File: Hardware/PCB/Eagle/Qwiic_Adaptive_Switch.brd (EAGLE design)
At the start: 41.9 x 30.5 mm, 18 parts, among them J2 J2, SW1 CUI_SJ1-3513, SW2 CUI_SJ1-3513

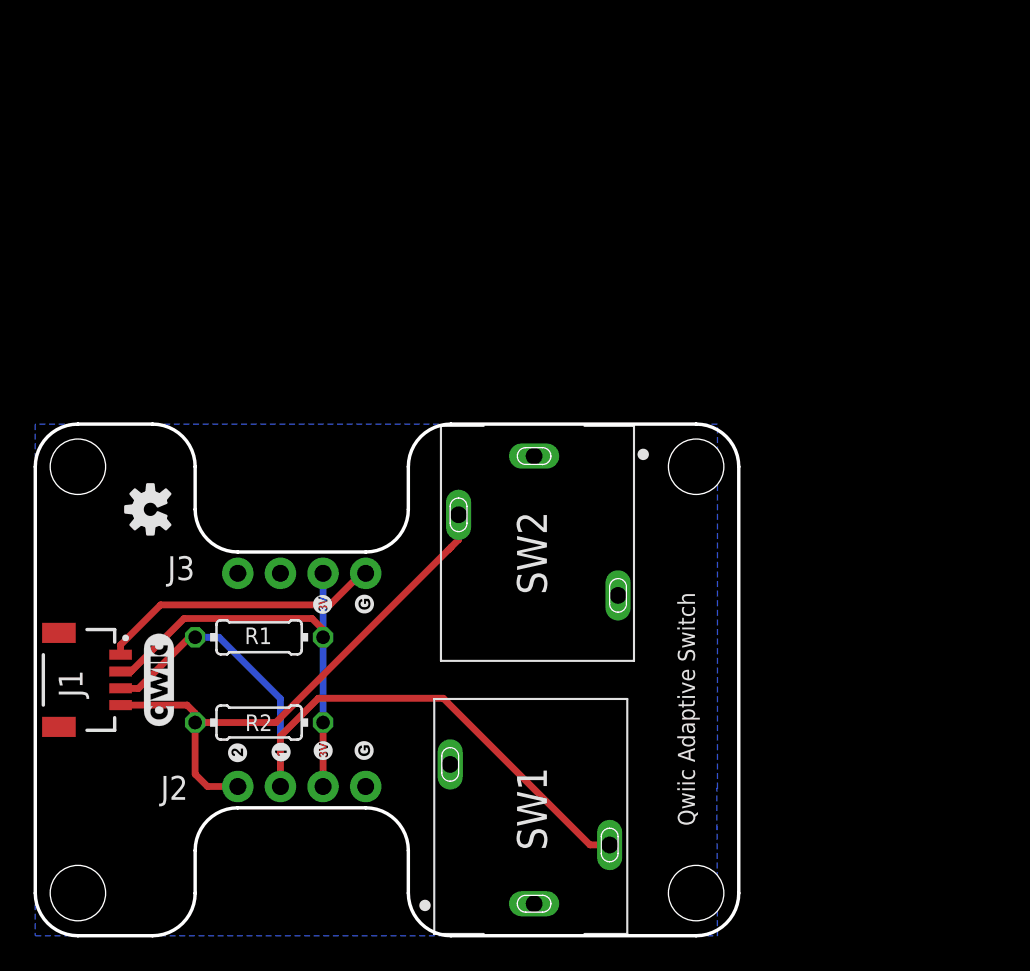
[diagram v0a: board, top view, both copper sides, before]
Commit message: Added Single and I2C BOM files
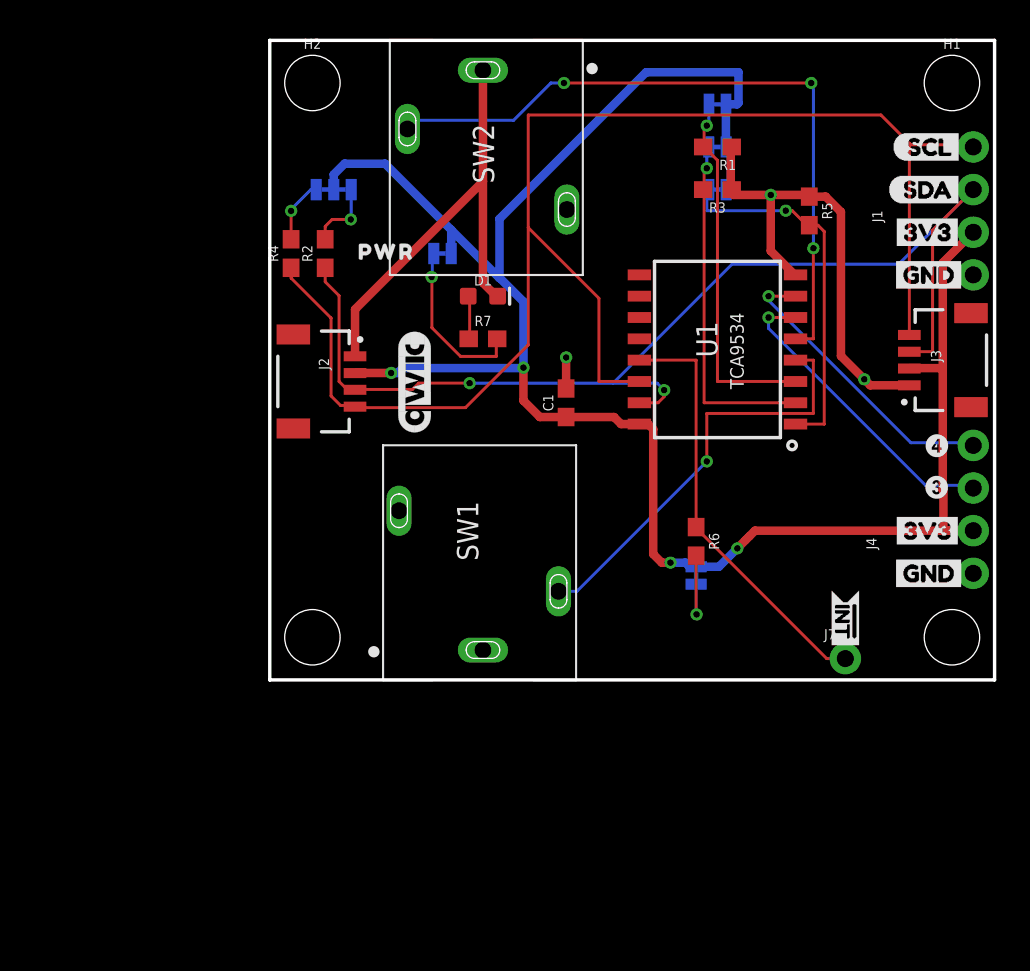
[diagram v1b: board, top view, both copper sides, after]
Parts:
- removed JP1, JP2: STAND-OFF, SparkFun-Hardware:STAND-OFF
- removed U$45: (no value), Labels:GND-03
- removed U$47: (no value), SDA:SDA0
- removed U$48: (no value), Labels:SCK-[)-03
- removed U$55: (no value), SparkFun-Aesthetics:QWIIC_5.5MM
- added ADR0, ADR1, INT, PWR: JUMPER-SMT_2_NC_TRACE_SILK, SparkFun-Jumpers:SMT-JUMPER_2_NC_TRACE_SILK
- added ADR2: JUMPER-SMT_2_NC_TRACE_NO-SILK, SparkFun-Jumpers:SMT-JUMPER_2_NC_TRACE_NO-SILK
- added C1: 0.1uF, SparkFun-Capacitors:0603
- added D1: RED, SparkFun-LED:LED-0603
- added H1, H2: STAND-OFF, SparkFun-Hardware:STAND-OFF
- added I2C: JUMPER-SMT_3_2-NC_TRACE_SILK, SparkFun-Jumpers:SMT-JUMPER_3_2-NC_TRACE_SILK
- added J4: (no value), SparkFun-Connectors:1X04_NO_SILK
- added J7: (no value), SparkFun-Connectors:1X01_NO_SILK
- added LOGO1: OSHW-LOGOMINI, SparkFun-Aesthetics:OSHW-LOGO-MINI
- added R3, R4, R5: 2.2k, SparkFun-Resistors:0603
- added R6: 10k, SparkFun-Resistors:0603
- added R7: 1k, SparkFun-Resistors:0603
- added U$10: (no value), buzzard_labels (44):SDA5
- added U$11: (no value), output:#ADR2#0
- added U$15: (no value), output:#ADR0#0
- added U$2, U$25, U$7: (no value), buzzard_labels (44):GND4
- added U$21: (no value), SparkFun-Aesthetics:QWIIC_6MM
- added U$22: (no value), buzzard_labels (54):#INT0
- added U$23: (no value), buzzard_labels (51):SCL0
- added U$24: (no value), buzzard_labels (51):SDA1
- added U$26, U$3, U$4: (no value), buzzard_labels (44):3V33
- added U$34: (no value), output:PWR0
- added U$39: (no value), output:#PWR#0
- added U$5: (no value), output:#ADR1#0
- added U$9: (no value), buzzard_labels (44):SCL6
- added U1: TCA9534, SparkFun-IC-Conversion:16SOIC
- J1: device SparkFun-Connectors:JST04_1MM_RA -> SparkFun-Connectors:1X04_NO_SILK
- J2: value J2 -> QWIIC; device SparkFun-Connectors:1X04_NO_SILK -> SparkFun-Connectors:JST04_1MM_RA
- J3: value (none) -> QWIIC; device SparkFun-Connectors:1X04_NO_SILK -> SparkFun-Connectors:JST04_1MM_RA
- JP3, JP4: device SparkFun-Hardware:STAND-OFF -> SparkFun:STAND-OFF
- R1, R2: value (none) -> 2.2k; device MMC Eagle:RESISTOR_0205/7 -> SparkFun-Resistors:0603
- U$1: device SparkFun-Aesthetics:OSHW-LOGO-S -> SparkFun-Buzzard:I2C
- U$12: device Labels:3V3-03 -> output:#INT#0
- U$13: device SparkFun-Aesthetics:OSHW-LOGO-S -> buzzard_labels (52):#INT0
- moved J1 56.2 mm to (41.9, 24.1), turned to 90 degrees
- moved U$13 42.3 mm to (34.3, 1.40)
- moved J3 42.0 mm to (38.1, 19.1), turned to 90 degrees
- moved R1 40.0 mm to (26.7, 31.8), turned to 180 degrees
- moved R2 28.2 mm to (3.30, 25.4), turned to 90 degrees
- moved J2 25.1 mm to (5.08, 17.8), turned to 270 degrees
- moved U$1 24.5 mm to (5.59, 31.1), flipped to the bottom, turned to 0 degrees
- moved U$12 23.7 mm to (23.6, 6.35), turned to 0 degrees
- moved SW2 23.2 mm to (12.7, 36.3)
- moved JP4 18.3 mm to (40.6, 2.54)
- moved JP3 17.3 mm to (2.54, 2.54)
- moved SW1 15.4 mm to (12.7, 1.78)
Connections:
- removed net SCL/SCK: J1.4, J2.1, R2.1, SW2.2
- removed net SDA/MOSI: J1.3, J2.2, R1.1, SW1.2
- new net !INT: J7.1, R6.1, U1.13
- new net ADR0: ADR0.1, R5.2, U1.1
- new net ADR1: ADR1.1, R3.2, U1.2
- new net ADR2: ADR2.1, R1.2, U1.3
- new net N$1: INT.1, R6.2
- new net N$2: D1.A, R7.1
- new net N$3: PWR.1, R7.2
- new net P0: SW1.2, U1.4
- new net P1: SW2.2, U1.5
- new net P2: J4.3, U1.6
- new net P3: J4.4, U1.7
- new net SCL: J1.4, J2.4, J3.4, R4.1, U1.14
- new net SCL_PU1: I2C.1, R2.2
- new net SDA: J1.3, J2.3, J3.3, R2.1, U1.15
- new net SDA_PU1: I2C.3, R4.2
- net 3.3V: now also ADR0.2, ADR1.2, ADR2.2, C1.1, I2C.2, INT.2, J2.2, J3.2, J4.2, PWR.2, U1.16; no longer J2.3, J3.3, R1.2, R2.2
- net GND: now also C1.2, D1.C, J2.1, J3.1, J4.1, R1.1, R3.1, R5.1, U1.8; no longer J2.4, J3.4
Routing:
- net 3.3V: track 26.8 -> 121.2 mm, vias 0 -> 4
- net SCL: track 0.00 -> 87.9 mm
- net SDA: track 0.00 -> 67.3 mm, vias 0 -> 2
- net SDA/MOSI: track 44.7 -> 0.00 mm
- net P1: track 0.00 -> 41.6 mm, vias 0 -> 3
- net GND: track 17.0 -> 58.0 mm, vias 0 -> 3
- net SCL/SCK: track 32.8 -> 0.00 mm
- net !INT: track 0.00 -> 25.5 mm
- net P0: track 0.00 -> 25.5 mm, vias 0 -> 1
- net ADR0: track 0.00 -> 22.1 mm, vias 0 -> 1
- net ADR2: track 0.00 -> 21.7 mm, vias 0 -> 1
- net ADR1: track 0.00 -> 20.9 mm, vias 0 -> 1
- net P2: track 0.00 -> 18.4 mm, vias 0 -> 1
- net P3: track 0.00 -> 17.6 mm, vias 0 -> 1
- net N$3: track 0.00 -> 10.1 mm, vias 0 -> 1
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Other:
- board size 41.9 x 30.5 mm -> 43.2 x 38.1 mm
- board text added: "I2C"
- board text added: "Qwiic-Adaptive-Switch"
- board text removed: "Qwiic Adaptive Switch"

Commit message: Updated design
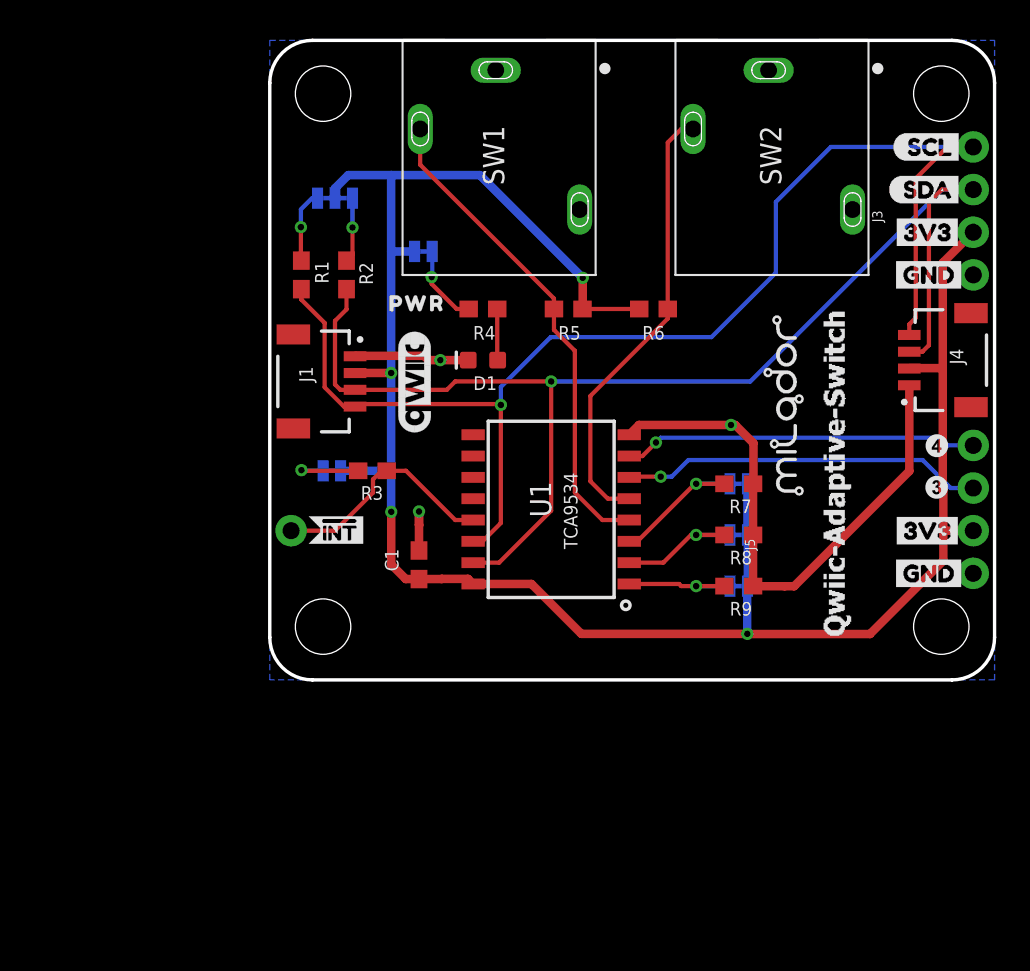
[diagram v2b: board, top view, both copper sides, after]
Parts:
- removed J7: (no value), SparkFun-Connectors:1X01_NO_SILK
- added J5: (no value), SparkFun-Connectors:1X04_NO_SILK
- added R8, R9: 2.2k, SparkFun-Resistors:0603
- added U$14: (no value), buzzard_labels (44):GND4
- added U$16, U$19: (no value), milador:MILADOR_QWIIC_SWITCH
- added U$17: MILADOR-SWITCH-NAME-SW1, milador:SWITCH-SW1
- added U$18: MILADOR-SWITCH-NAME-SW2, milador:SWITCH-SW2
- added U$20, U$6: MILADOR-LOGO-, milador:MILADOR_LOGO1
- added U$8: (no value), buzzard_labels (44):3V33
- ADR2: value JUMPER-SMT_2_NC_TRACE_NO-SILK -> JUMPER-SMT_2_NC_TRACE_SILK; device SparkFun-Jumpers:SMT-JUMPER_2_NC_TRACE_NO-SILK -> SparkFun-Jumpers:SMT-JUMPER_2_NC_TRACE_SILK
- J1, J4: value (none) -> QWIIC; device SparkFun-Connectors:1X04_NO_SILK -> SparkFun-Connectors:JST04_1MM_RA
- J2: value QWIIC -> (none); device SparkFun-Connectors:JST04_1MM_RA -> SparkFun-Connectors:1X01_NO_SILK
- J3: value QWIIC -> (none); device SparkFun-Connectors:JST04_1MM_RA -> SparkFun-Connectors:1X04_NO_SILK
- R3, R5: value 2.2k -> 10k
- R4: value 2.2k -> 1k
- R6: value 10k -> 10K
- R7: value 1k -> 2.2k
- moved J1 37.4 mm to (5.08, 17.8), turned to 270 degrees
- moved SW1 34.6 mm to (13.5, 36.3), turned to 270 degrees
- moved U$22 32.4 mm to (2.05, 8.93), turned to 0 degrees
- moved U$13 29.0 mm to (6.28, 8.93), turned to 0 degrees
- moved R3 26.5 mm to (6.11, 12.5)
- moved R1 25.9 mm to (1.88, 24.1), turned to 90 degrees
- moved ADR0 23.7 mm to (27.9, 5.59)
- moved U$15 23.6 mm to (34.0, 5.59)
- moved ADR1 23.1 mm to (27.9, 8.64)
- moved U$5 23.1 mm to (34.0, 8.64)
- moved ADR2 22.6 mm to (27.9, 11.7)
- moved U$11 22.6 mm to (34.0, 11.7)
- moved INT 22.6 mm to (3.70, 12.5), turned to 180 degrees
- moved R7 17.5 mm to (27.9, 11.7), turned to 180 degrees
- moved SW2 17.0 mm to (29.7, 36.3)
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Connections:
- net !INT: now also J2.1, R3.1; no longer J7.1, R6.1
- net 3.3V: now also J5.2, R5.2, R6.2; no longer J2.2
- net ADR0: now also R9.2; no longer R5.2
- net ADR1: now also R8.2; no longer R3.2
- net ADR2: now also R7.2; no longer R1.2
- net GND: now also J5.1, R7.1, R8.1, R9.1; no longer J2.1, R1.1, R3.1, R5.1
- net N$1: now also R3.2; no longer R6.2
- net N$2: now also R4.1; no longer R7.1
- net N$3: now also R4.2; no longer R7.2
- net P0: now also R5.1
- net P1: now also R6.1
- net P2: now also J5.3; no longer J4.3
- net P3: now also J5.4; no longer J4.4
- net SCL: now also J4.4, R1.1; no longer J2.4, R4.1
- net SDA: now also J4.3; no longer J2.3
- net SDA_PU1: now also R1.2; no longer R4.2
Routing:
- net P1: track 41.6 -> 26.7 mm, vias 3 -> 0
- net ADR0: track 22.1 -> 7.75 mm
- net GND: track 58.0 -> 43.9 mm
- net ADR2: track 21.7 -> 9.12 mm
- net ADR1: track 20.9 -> 8.38 mm
- net !INT: track 25.5 -> 14.0 mm
- net SCL: track 87.9 -> 78.0 mm, vias 0 -> 1
- net SDA: track 67.3 -> 76.2 mm, vias 2 -> 1
- net N$3: track 10.1 -> 4.79 mm
- net P0: track 25.5 -> 29.4 mm, vias 1 -> 0
- net P3: track 17.6 -> 21.1 mm
- net P2: track 18.4 -> 21.6 mm
- net 3.3V: track 121.2 -> 122.8 mm
- net N$1: track 5.32 -> 4.70 mm
- net SDA_PU1: track 3.77 -> 4.33 mm
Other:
- outline, holes or cut-outs redrawn
- board text removed: "I2C"
- board text removed: "Qwiic-Adaptive-Switch"

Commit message: Updated the design.
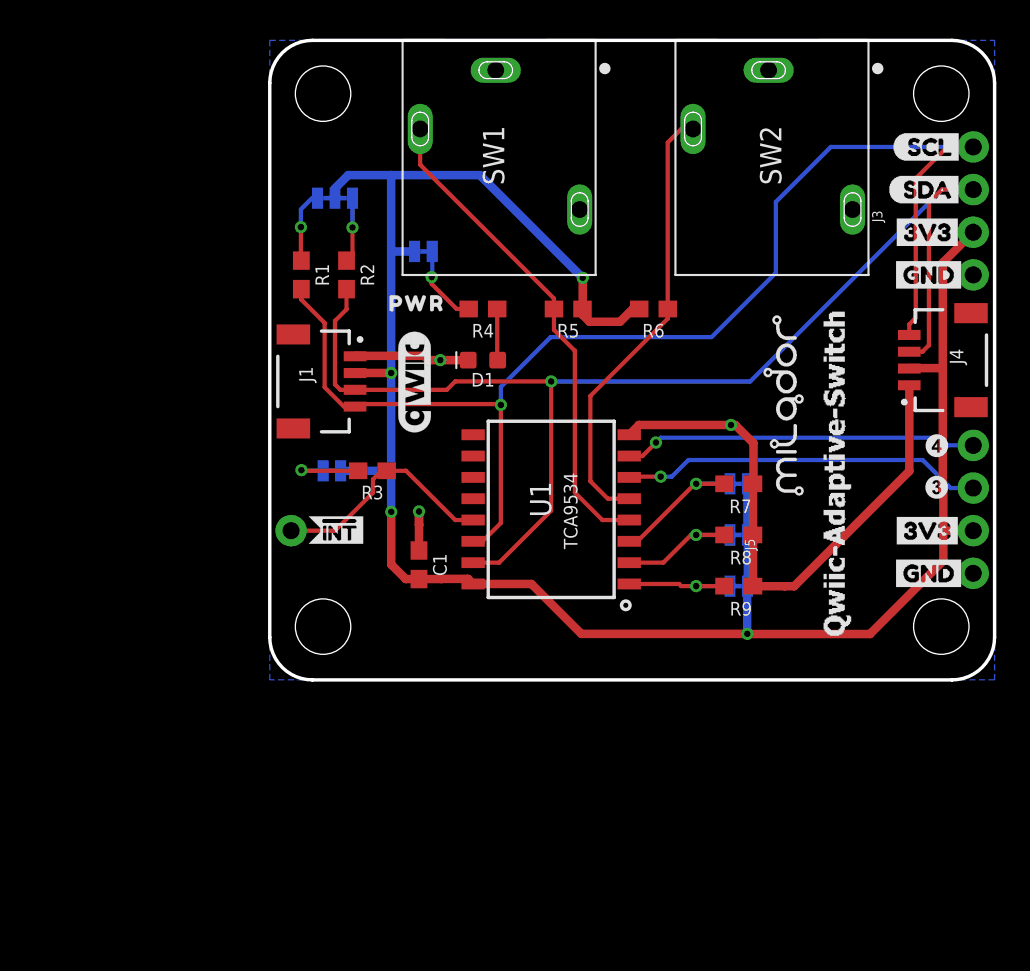
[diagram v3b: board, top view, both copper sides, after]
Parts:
- removed LOGO1: OSHW-LOGOMINI, SparkFun-Aesthetics:OSHW-LOGO-MINI
- ADR0, ADR1, ADR2, INT, PWR: value JUMPER-SMT_2_NC_TRACE_SILK -> JUMPERS-SMT_2_NC_TRACE_SILK; device SparkFun-Jumpers:SMT-JUMPER_2_NC_TRACE_SILK -> milador_SMD:JUMPERS_SMT-JUMPER_2_NC_TRACE_SILK
- C1: device SparkFun-Capacitors:0603 -> milador_SMD:0603
- D1: device SparkFun-LED:LED-0603 -> milador_SMD:LED-0603
- I2C: value JUMPER-SMT_3_2-NC_TRACE_SILK -> JUMPERS_JUMPER-SMT_3_2-NC_TRACE_SILK; device SparkFun-Jumpers:SMT-JUMPER_3_2-NC_TRACE_SILK -> milador_SMD:JUMPERS_SMT-JUMPER_3_2-NC_TRACE_SILK
- J1, J4: value QWIIC -> QWIIC_RIGHT_ANGLE; device SparkFun-Connectors:JST04_1MM_RA -> milador_SMD:CONNECTORS_JST04_1MM_RA
- J2: device SparkFun-Connectors:1X01_NO_SILK -> milador:CONNECTORS_1X01_NO_SILK
- J3, J5: device SparkFun-Connectors:1X04_NO_SILK -> milador:CONNECTORS_1X04_NO_SILK
- R1, R2, R3, R4, R5, R6, R7, R8, R9: device SparkFun-Resistors:0603 -> milador_SMD:0603
- U1: device SparkFun-IC-Conversion:16SOIC -> milador_SMD:16SOIC
- moved U$20 0.13 mm to (26.3, 18.4)
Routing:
- net 3.3V: track 122.8 -> 123.7 mm
- net SDA: track 76.2 -> 75.5 mm

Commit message: Updated the design - Stable design
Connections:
- net GND: now also SW1.3, SW2.3
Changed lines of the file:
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@@
 <drawing>
 <settings>
-<setting alwaysvectorfont="no"/>
+<setting alwaysvectorfont="yes"/>
 <setting keepoldvectorfont="yes"/>
 <setting verticaltext="up"/>
@@
 </layers>
 <board>
-<fusionsync huburn="a.cGVyc29uYWw6dWUyYWQxOTI2" projecturn="a.cGVyc29uYWw6dWUyYWQxOTI2IzIwMjEwMTA3MzY5MTI4NTU2" f3durn="urn:adsk.wipprod:dm.lineage:iqi4HTDMROu8o-H5T5Jb5A" pcbguid="" lastpulledtime="" lastsyncedchangeguid="" latestrevisionid="083c6886-957b-4a1f-a4c9-710898d37edb" lastsyncedrevisionid="083c6886-957b-4a1f-a4c9-710898d37edb" lastboardhashguid="66578006-9f20-48b5-7580-e67f18d5f324" lastpushedtime="2021-06-05T03:26:52Z" linktopcb3d="true"/>
+<fusionsync huburn="a.cGVyc29uYWw6dWUyYWQxOTI2" projecturn="a.cGVyc29uYWw6dWUyYWQxOTI2IzIwMjEwMTA3MzY5MTI4NTU2" f3durn="urn:adsk.wipprod:dm.lineage:iqi4HTDMROu8o-H5T5Jb5A" pcbguid="" lastpulledtime="" lastsyncedchangeguid="" latestrevisionid="a4c49c8c-9ee0-401c-9360-ad30710fd072" lastsyncedrevisionid="a4c49c8c-9ee0-401c-9360-ad30710fd072" lastboardhashguid="7686bb73-5b86-c421-8fb9-e947596aed68" lastpushedtime="2021-06-23T00:17:49Z" linktopcb3d="true"/>
 <plain>
 <wire x1="0" y1="0" x2="0" y2="25.4" width="0.2032" layer="52"/>
@@
 <wire x1="38.1" y1="12.440921875" x2="31.238096875" y2="5.57901875" width="0.508" layer="1"/>
 <wire x1="31.238096875" y1="5.57901875" x2="30.6705" y2="5.57901875" width="0.508" layer="1"/>
+<contactref element="SW2" pad="3"/>
+<contactref element="SW1" pad="3"/>
 </signal>
 <signal name="SCL_PU1">
